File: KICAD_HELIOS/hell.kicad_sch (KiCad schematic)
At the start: 43 parts, among them J101 NC3FAAH, J102 NC3MAAH, J103 ecran, J104 Conn_ST_STDC14, J105 Conn_01x02, SW101 SW_Push, SW102 SW_Push, SW103 SW_Push, U101 R-78B5.0-2.0, U102 AMS1117-3.3, U103 MAX485E, U104 STM32F103C6Tx

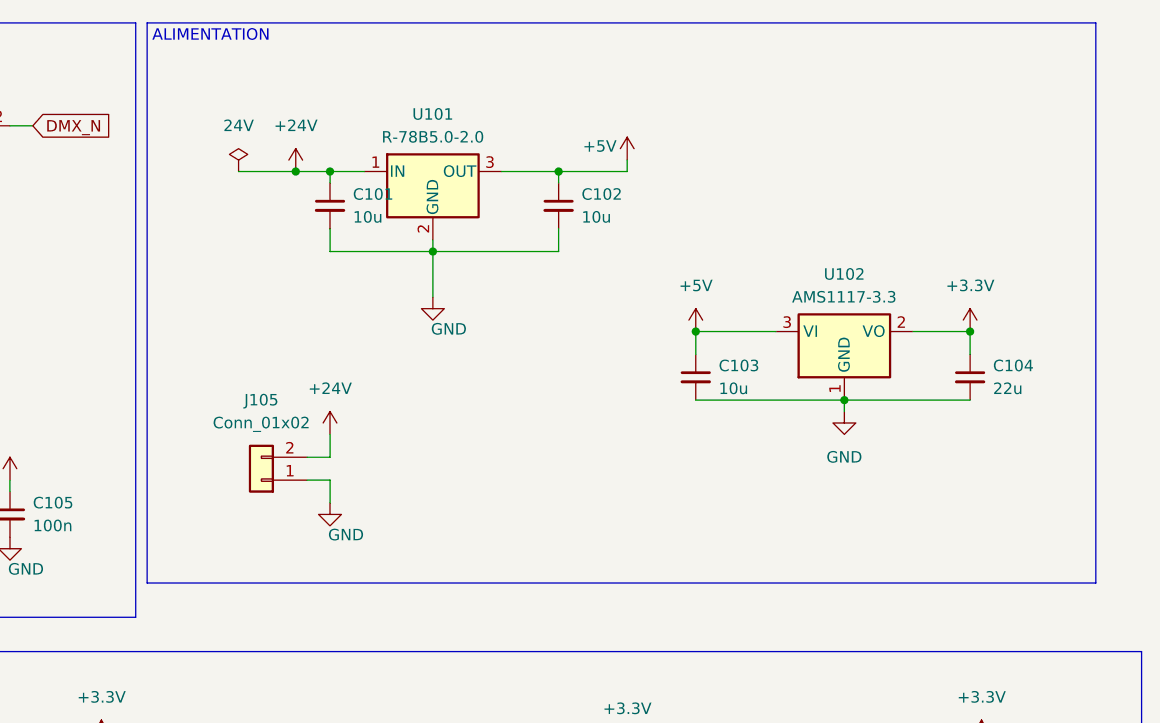
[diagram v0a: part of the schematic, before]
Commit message: PCB
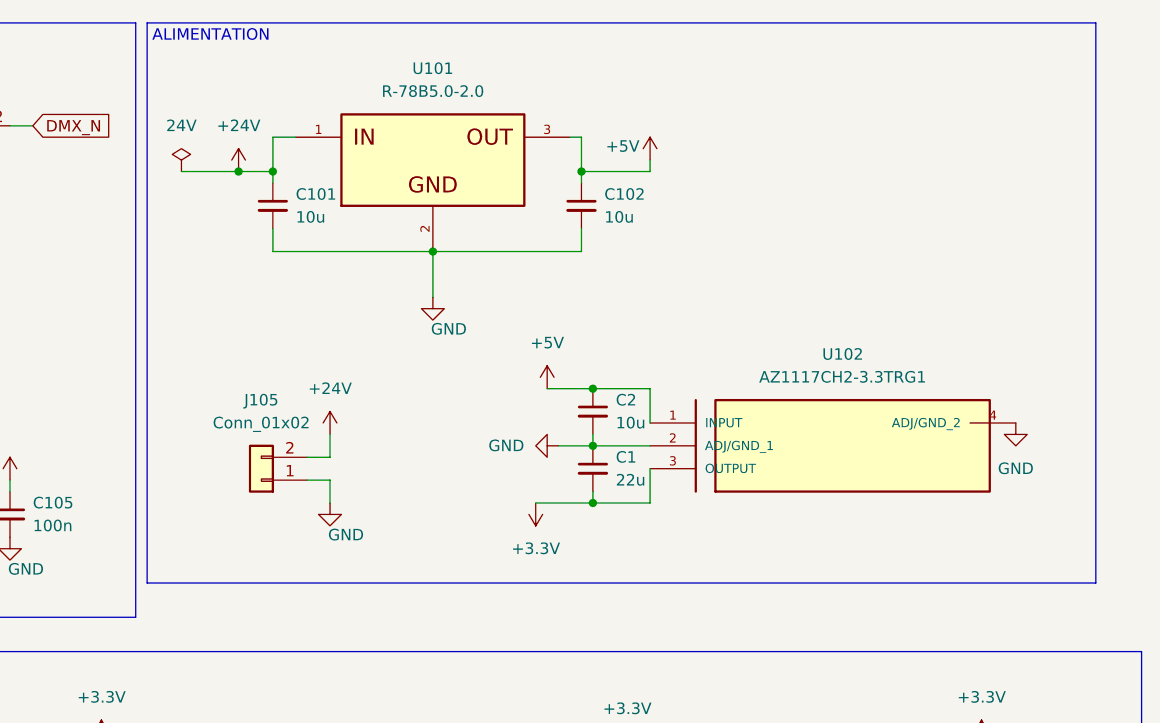
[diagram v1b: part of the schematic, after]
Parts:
- removed C103: 10u, Capacitor_SMD:C_0603_1608Metric, symbol Device:C_Small
- removed C104: 22u, Capacitor_SMD:C_0805_2012Metric, symbol Device:C_Small
- removed U101: R-78B5.0-2.0, Converter_DCDC:Converter_DCDC_RECOM_R-78B-2.0_THT, symbol Converter_DCDC:R-78B2.5-2.0
- removed U102: AMS1117-3.3, Package_TO_SOT_SMD:SOT-223-3_TabPin2, symbol Regulator_Linear:AMS1117-3.3
- added C1: 22u, Capacitor_SMD:C_0805_2012Metric, symbol Device:C_Small
- added C2: 10u, Capacitor_SMD:C_0603_1608Metric, symbol Device:C_Small
- added U101: R-78B5.0-2.0, WPME-FDSM_SIP-3:WPME-FDSM_173950536, symbol WPME-FDSM_SIP-3:WPME-FDSM_SIP-3
- added U102: AZ1117CH2-3.3TRG1, AZ1117CH2-3.3TRG1:SOT230P700X180-4N, symbol AZ1117CH2-3.3TRG1:AZ1117CH2-3.3TRG1
- U103: MPN (none) -> MAX485E
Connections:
- net +24V: now also U101.1
- net +3.3V: now also C1.2, U102.3 (OUTPUT)
- net +5V: now also C2.1, U101.3, U102.1 (INPUT)
- net GND: now also C1.1, C2.2, U101.2, U102.2 (ADJ/GND_1), U102.4 (ADJ/GND_2)
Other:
- moved on the sheet: C101, C102
